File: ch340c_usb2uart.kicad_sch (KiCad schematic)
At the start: 2 parts, among them J1 USB_A, U1 CH340C

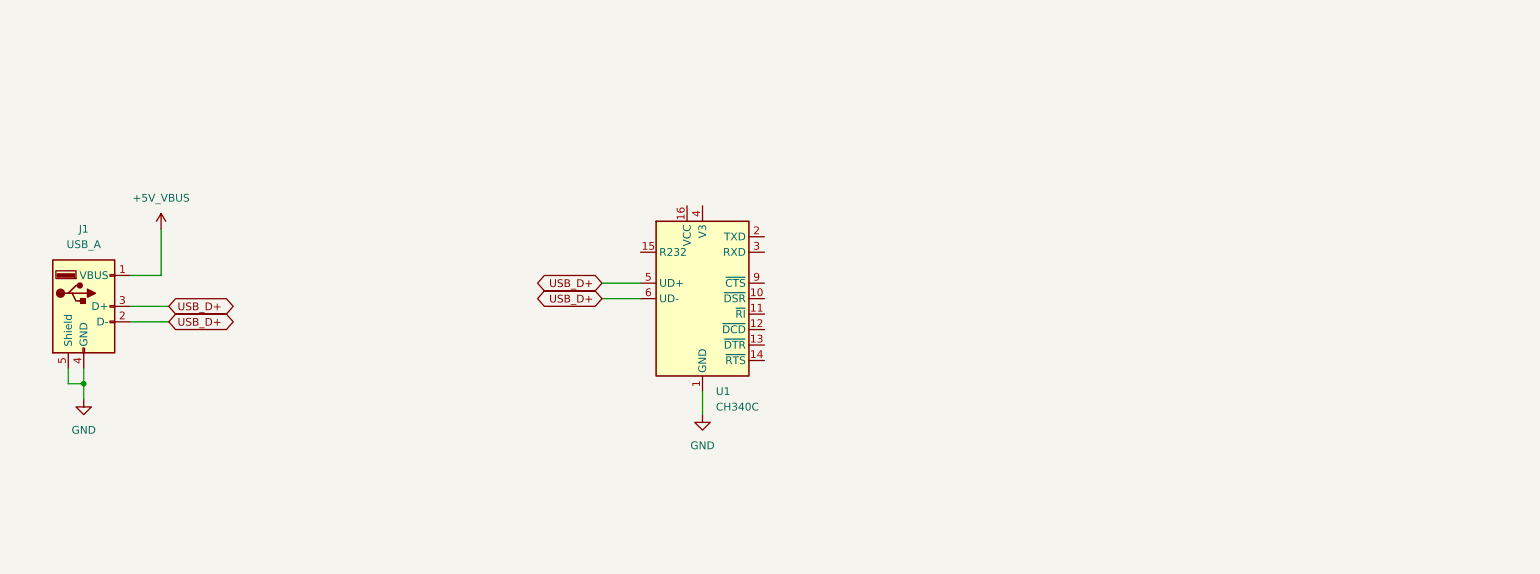
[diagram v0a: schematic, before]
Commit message: first commit
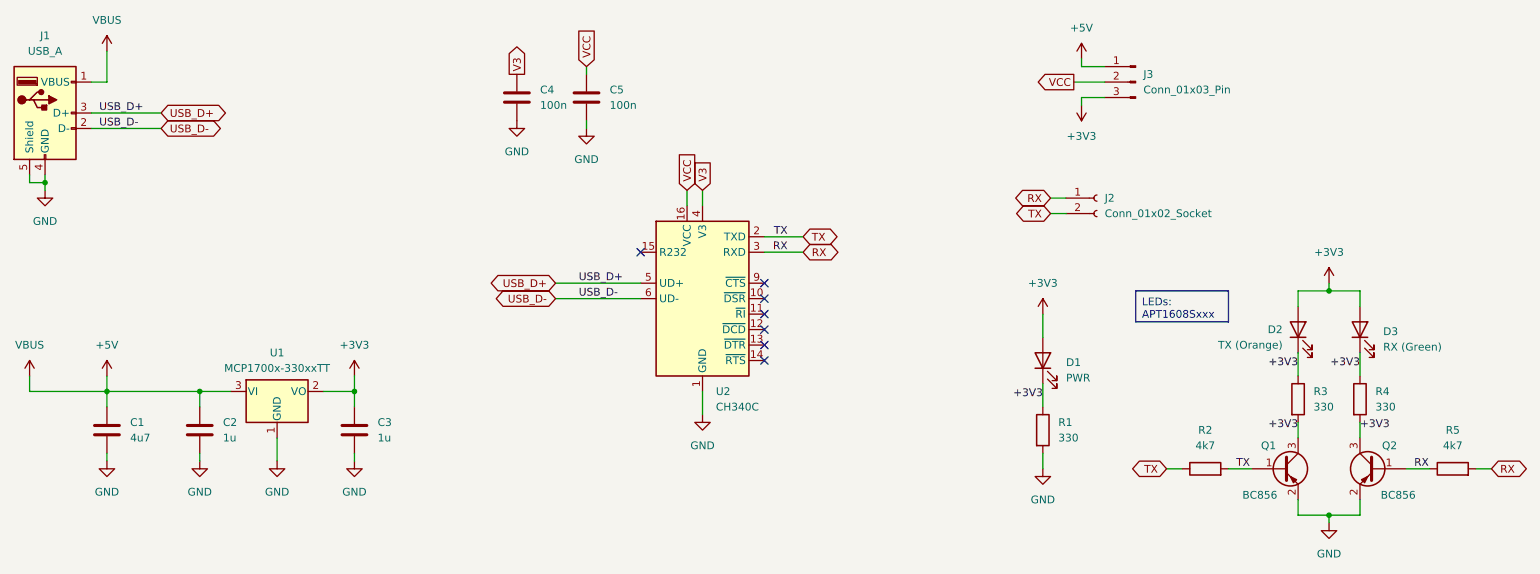
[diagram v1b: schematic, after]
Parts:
- added C1: 4u7, Capacitor_SMD:C_0603_1608Metric, symbol Device:C
- added C2, C3: 1u, Capacitor_SMD:C_0603_1608Metric, symbol Device:C
- added C4, C5: 100n, Capacitor_SMD:C_0603_1608Metric, symbol Device:C
- added D1: PWR, LED_SMD:LED_0603_1608Metric, symbol Device:LED
- added D2: TX (Orange), LED_SMD:LED_0603_1608Metric, symbol Device:LED
- added D3: RX (Green), LED_SMD:LED_0603_1608Metric, symbol Device:LED
- added J2: Conn_01x02_Socket, Connector_JST:JST_PH_S2B-PH-K_1x02_P2.00mm_Horizontal, symbol Connector:Conn_01x02_Socket
- added J3: Conn_01x03_Pin, Connector_PinHeader_2.54mm:PinHeader_1x03_P2.54mm_Vertical, symbol Connector:Conn_01x03_Pin
- added Q1, Q2: BC856, Package_TO_SOT_SMD:SOT-23, symbol Transistor_BJT:BC856
- added R1, R3, R4: 330, Resistor_SMD:R_0603_1608Metric, symbol Device:R
- added R2, R5: 4k7, Resistor_SMD:R_0603_1608Metric, symbol Device:R
- added U1: MCP1700x-330xxTT, Package_TO_SOT_SMD:SOT-23, symbol Regulator_Linear:MCP1700x-330xxTT
- J1: footprint (none) -> Connector_USB:USB_A_Molex_48037-2200_Horizontal
- renumbered U1 to U2
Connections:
- net GND: now also C1.2, C2.2, C3.2, C4.2, C5.2, Q1.2 (E), Q2.2 (E), R1.2, U1.1 (GND)
- net USB_D+: no longer J1.2 (D-), U2.6 (UD-)
- net VCC: now reaches U2.16 (VCC)
- net VCC: now also C5.1, J3.2 (Pin_2)
- net TX: now reaches U2.2 (TXD)
- net TX: now also J2.2 (Pin_2), Q1.1 (B), R2.1, R2.2
- net RX: now reaches U2.3 (RXD)
- net RX: now also J2.1 (Pin_1), Q2.1 (B), R5.1, R5.2
- net V3: now reaches U2.4 (V3)
- net V3: now also C4.1
- net +5V_VBUS renamed +5V
- net +5V: now also C1.1, C2.1, J3.1 (Pin_1), U1.3 (VI)
- new net +3V3: C3.1, D1.1 (K), D1.2 (A), D2.1 (K), D2.2 (A), D3.1 (K), D3.2 (A), J3.3 (Pin_3), Q1.3 (C), Q2.3 (C), R1.1, R3.1, R3.2, R4.1, R4.2, U1.2 (VO)
- new net USB_D-: J1.2 (D-), U2.6 (UD-)
- no-connect marks 0 -> 7
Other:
- moved on the sheet: J1
